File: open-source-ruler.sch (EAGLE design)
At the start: 59 parts, among them IC1 LT1007CS8, IC2 FT232RLSSOP, IC3 MDC3105DMT1, IC4 XMEGA16A4A, Q4 ASF1, U1 V_REG_317DPACK, U2 ATMEGA168, U3 ATMEGA168MLF, U4 7432SE, X1 MINI-USB-UX60A-MB-5ST

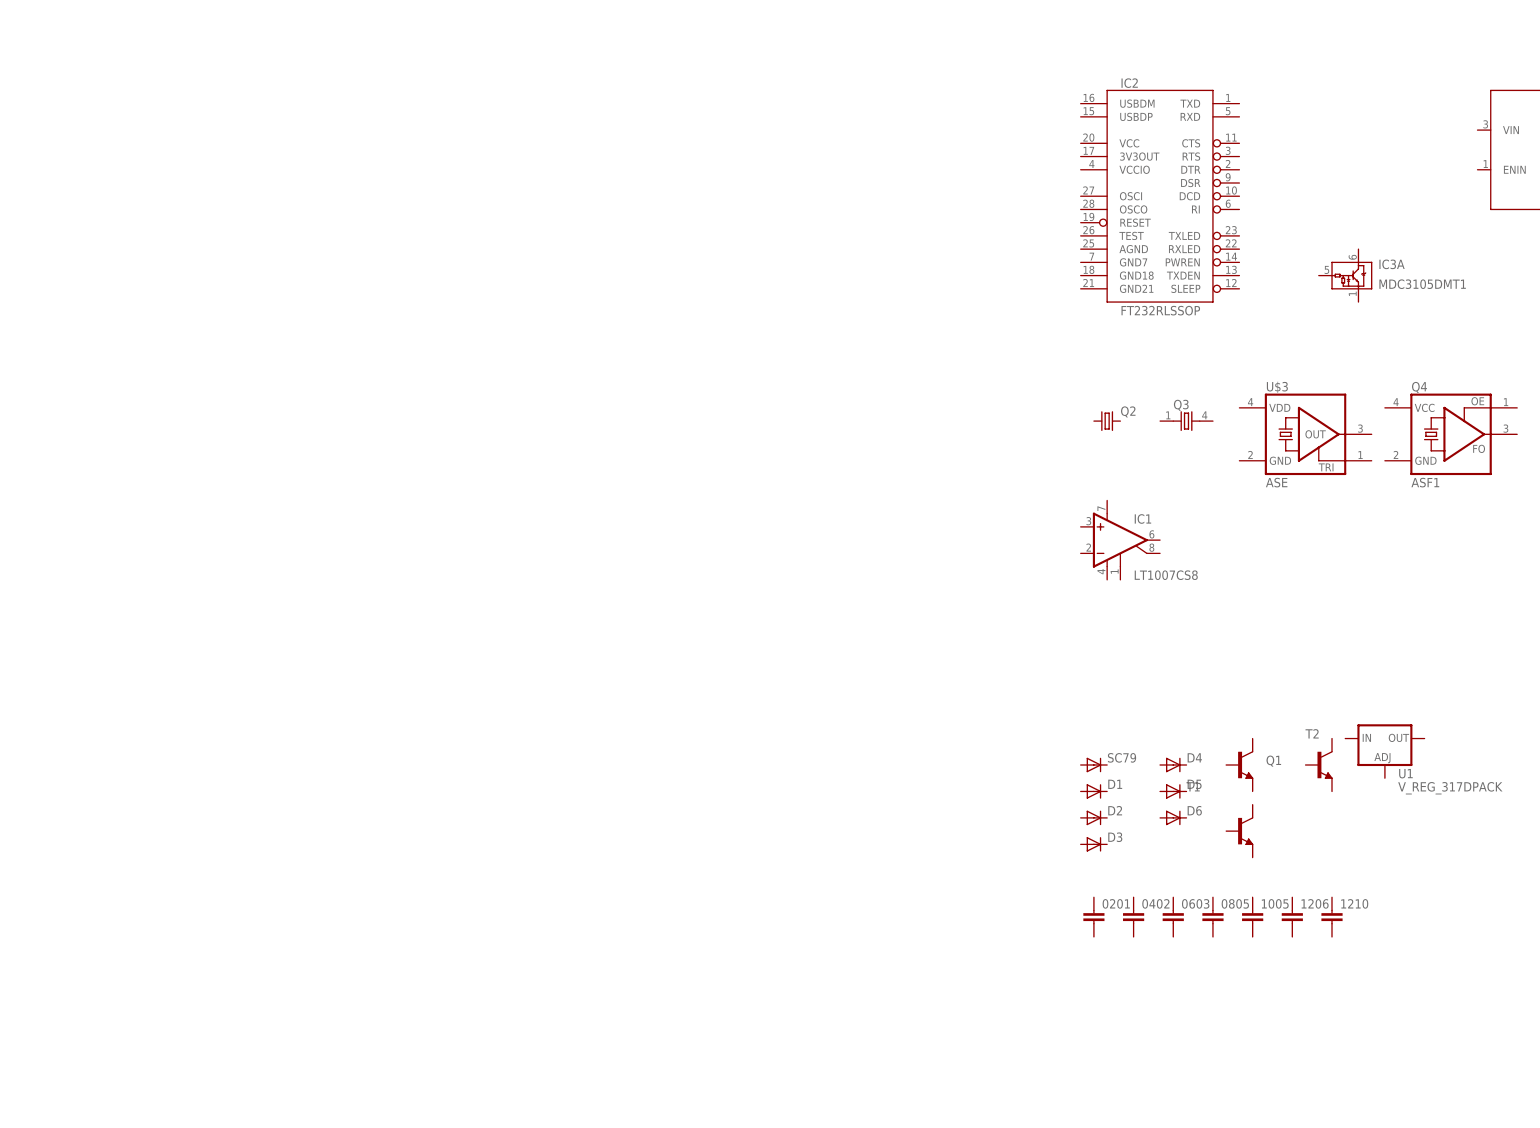
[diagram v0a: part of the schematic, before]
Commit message: Ready for release
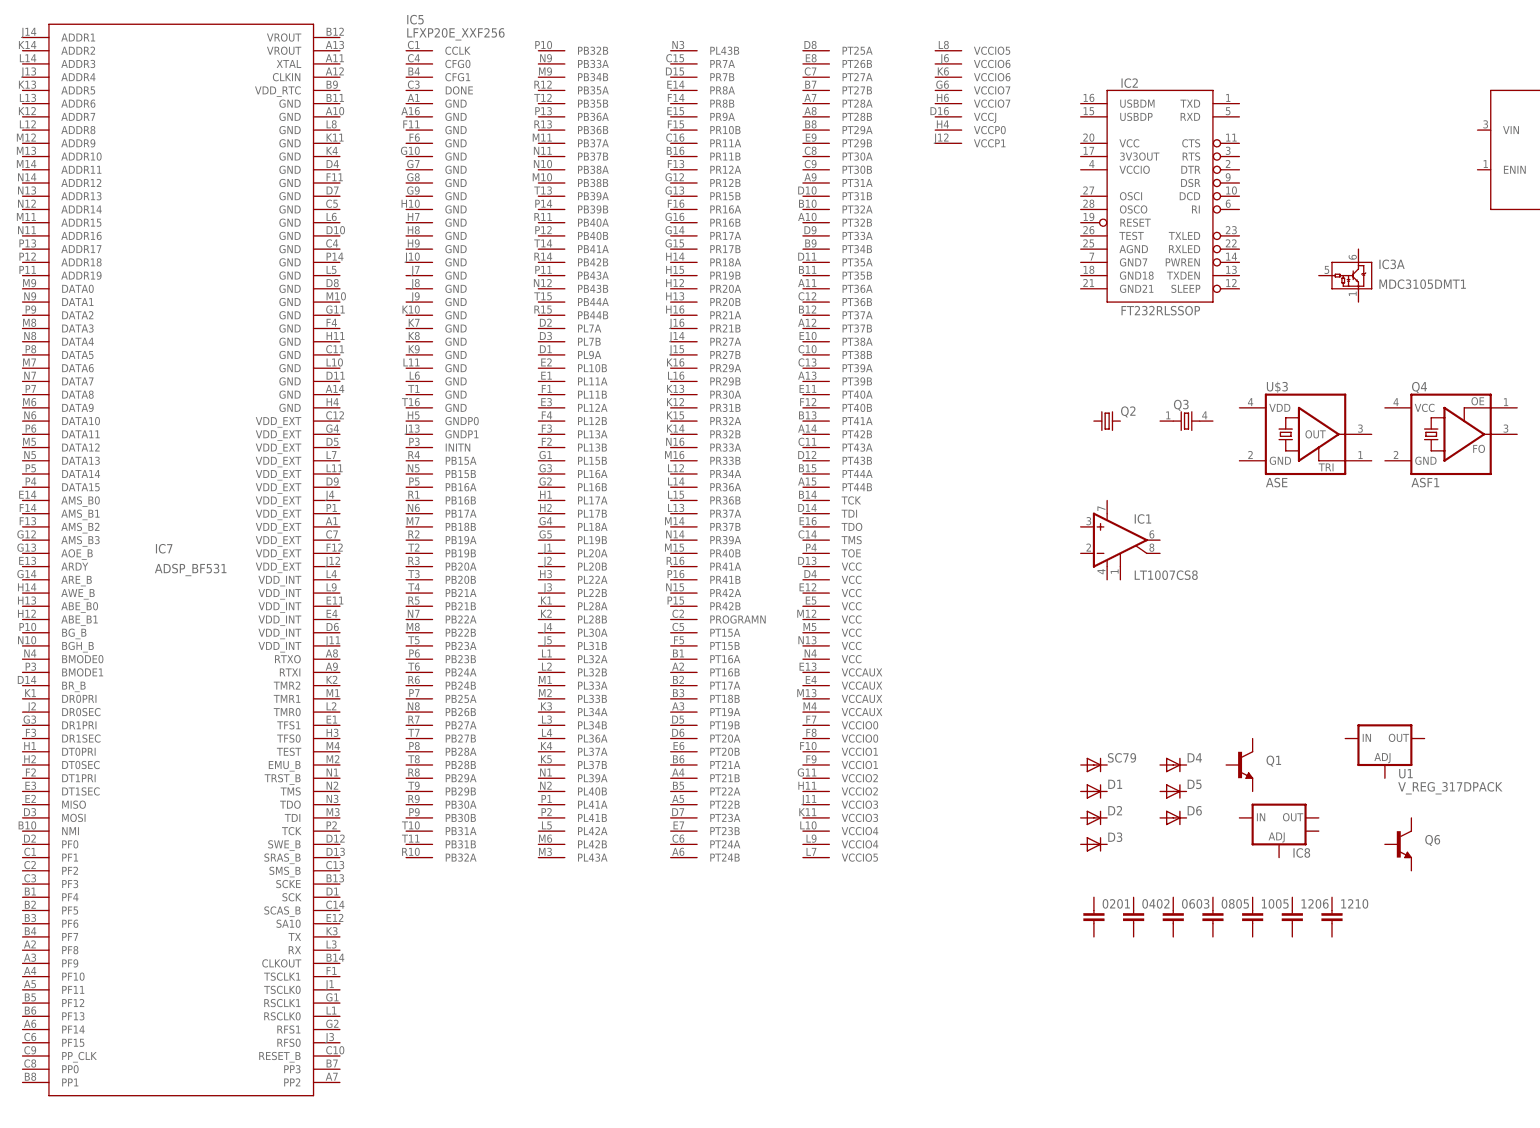
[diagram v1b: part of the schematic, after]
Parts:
- removed T1: (no value), transistor-neu-to92:-NPN-SOT223
- removed T2: (no value), transistor-neu-to92:-NPN-SOT89-BCE
- added IC5: LFXP20E_XXF256, lattice:LFXP20E_XXF256
- added IC7: ADSP_BF531, analog-devices:ADSP_BF531
- added IC8: (no value), SparkFun:V_REG_LM1117SOT223
- added Q6: (no value), SparkFun:TRANSISTOR_NPNSOT89
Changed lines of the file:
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@@
 <part name="D6" library="diode" deviceset="DIODE-" device="SMC"/>
 <part name="Q1" library="SparkFun" deviceset="TRANSISTOR_NPN" device="SOT23"/>
-<part name="T1" library="transistor-neu-to92" deviceset="*-NPN-" device="SOT223"/>
 <part name="U1" library="SparkFun" deviceset="V_REG_317" device="DPACK"/>
 <part name="IC1" library="linear" deviceset="LT10*" device="S8" technology="07C"/>
-<part name="T2" library="transistor-neu-to92" deviceset="*-NPN-" device="SOT89-BCE"/>
 <part name="IC2" library="SparkFun" deviceset="FT232RL" device="SSOP"/>
 <part name="IC3" library="on-semiconductor" deviceset="MDC3105DMT1" device=""/>
@@
 <part name="U$26" library="SparkFun" deviceset="U.FL" device=""/>
 <part name="S1" library="SparkFun" deviceset="SWITCH-MOMENTARY-2" device=""/>
+<part name="IC5" library="lattice" deviceset="LFXP20E_XXF256" device=""/>
+<part name="IC7" library="analog-devices" deviceset="ADSP_BF531" device=""/>
+<part name="IC8" library="SparkFun" deviceset="V_REG_LM1117" device="SOT223"/>
+<part name="Q6" library="SparkFun" deviceset="TRANSISTOR_NPN" device="SOT89"/>
 </parts>
 <sheets>
@@
 <instance part="D6" gate="G$1" x="25.4" y="30.48"/>
 <instance part="Q1" gate="G$1" x="38.1" y="40.64"/>
-<instance part="T1" gate="G$1" x="38.1" y="27.94"/>
 <instance part="U1" gate="G$1" x="66.04" y="45.72"/>
 <instance part="IC1" gate="G$1" x="15.24" y="83.82"/>
-<instance part="T2" gate="G$1" x="53.34" y="40.64" smashed="yes">
-<attribute name="NAME" x="50.8" y="45.72" size="1.778" layer="95"/>
-<attribute name="VALUE" x="43.18" y="45.72" size="1.778" layer="96"/>
-</instance>
 <instance part="IC2" gate="G$1" x="22.86" y="149.86"/>
 <instance part="IC3" gate="A" x="58.42" y="134.62"/>
@@
 <instance part="U$26" gate="G$1" x="190.5" y="58.42"/>
 <instance part="S1" gate="G$1" x="165.1" y="86.36"/>
+<instance part="IC5" gate="G$1" x="-66.04" y="96.52"/>
+<instance part="IC7" gate="G$1" x="-195.58" y="-22.86"/>
+<instance part="IC8" gate="G$1" x="45.72" y="30.48"/>
+<instance part="Q6" gate="G$1" x="68.58" y="25.4"/>
 </instances>
 <busses>

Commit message: Ready to prototype
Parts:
- removed U$1: OSHW-LOGOS, SparkFun:OSHW-LOGOS
- added D7: (no value), diode:DIODE-MELF-MLL41
- added D8: (no value), diode:DIODE-MINIMELF
- added IC9: (no value), linear:LM2596S
- added U$27: LOGO_SMALL, my:LOGO_SMALL
- added U$28: OSHW-LOGOM, SparkFun:OSHW-LOGOM
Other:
- moved on the sheet: IC1, IC2, IC3A, IC4, IC5, IC6, IC7, IC8, Q2, Q3, Q4, Q5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
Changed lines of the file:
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@@
 <part name="1206" library="rcl" deviceset="C-EU" device="C1206"/>
 <part name="1210" library="rcl" deviceset="C-EU" device="C1210"/>
-<part name="FRAME1" library="frames" deviceset="A4L-LOC" device=""/>
 <part name="SC79" library="diode" deviceset="DIODE-" device="SC79_INFINEON"/>
 <part name="D1" library="diode" deviceset="DIODE-" device="MICROMELF-R"/>
@@
 <part name="Q5" library="crystal" deviceset="CRYSTAL" device="CTS406"/>
 <part name="QG1" library="crystal" deviceset="SM77H" device=""/>
-<part name="U$1" library="SparkFun" deviceset="OSHW-LOGO" device="S"/>
 <part name="U2" library="SparkFun" deviceset="ATMEGA168" device=""/>
 <part name="U3" library="SparkFun" deviceset="ATMEGA168" device="MLF"/>
@@
 <part name="IC8" library="SparkFun" deviceset="V_REG_LM1117" device="SOT223"/>
 <part name="Q6" library="SparkFun" deviceset="TRANSISTOR_NPN" device="SOT89"/>
+<part name="D7" library="diode" deviceset="DIODE-" device="MELF-MLL41"/>
+<part name="D8" library="diode" deviceset="DIODE-" device="MINIMELF"/>
+<part name="IC9" library="linear" deviceset="LM2596S" device=""/>
+<part name="U$27" library="my" deviceset="LOGO_SMALL" device=""/>
+<part name="U$28" library="SparkFun" deviceset="OSHW-LOGO" device="M"/>
+<part name="FRAME2" library="frames" deviceset="DINA3_L" device=""/>
 </parts>
 <sheets>
 <sheet>
 <plain>
-<text x="165.1" y="5.08" size="2.1844" layer="94" font="vector">hemal@black-electronics.com</text>
-<text x="223.52" y="30.48" size="2.54" layer="91">CC-BY-SA 3.0</text>
-<text x="165.1" y="10.16" size="2.54" layer="94" font="vector">Hemal Chevli</text>
+<text x="292.1" y="17.78" size="2.1844" layer="94" font="vector">hemal@black-electronics.com</text>
+<text x="348.742" y="126.492" size="2.54" layer="91">CC-BY-SA 3.0</text>
+<text x="292.1" y="22.86" size="2.54" layer="94" font="vector">Hemal Chevli</text>
 </plain>
 <instances>
@@
 <instance part="1206" gate="G$1" x="48.26" y="12.7"/>
 <instance part="1210" gate="G$1" x="55.88" y="12.7"/>
-<instance part="FRAME1" gate="G$1" x="0" y="0"/>
 <instance part="SC79" gate="G$1" x="10.16" y="40.64"/>
 <instance part="D1" gate="G$1" x="10.16" y="35.56"/>
@@
 <instance part="D6" gate="G$1" x="25.4" y="30.48"/>
 <instance part="Q1" gate="G$1" x="38.1" y="40.64"/>
-<instance part="U1" gate="G$1" x="66.04" y="45.72"/>
-<instance part="IC1" gate="G$1" x="15.24" y="83.82"/>
-<instance part="IC2" gate="G$1" x="22.86" y="149.86"/>
-<instance part="IC3" gate="A" x="58.42" y="134.62"/>
-<instance part="U$2" gate="G$1" x="86.36" y="147.32"/>
-<instance part="Q2" gate="G$1" x="12.7" y="106.68"/>
-<instance part="Q3" gate="G$1" x="27.94" y="106.68"/>
-<instance part="U$3" gate="G$1" x="50.8" y="104.14"/>
-<instance part="Q4" gate="G$1" x="78.74" y="104.14"/>
-<instance part="Q5" gate="G$1" x="99.06" y="104.14"/>
-<instance part="QG1" gate="G$1" x="119.38" y="104.14"/>
-<instance part="U$1" gate="G$1" x="236.22" y="43.18"/>
-<instance part="U2" gate="G$1" x="162.56" y="142.24"/>
-<instance part="U3" gate="G$1" x="220.98" y="142.24"/>
-<instance part="U4" gate="G$1" x="213.36" y="86.36"/>
-<instance part="U$5" gate="G$1" x="114.3" y="55.88"/>
-<instance part="X1" gate="G$1" x="154.94" y="55.88" smashed="yes"/>
-<instance part="U$6" gate="G$1" x="284.48" y="165.1"/>
-<instance part="U$7" gate="G$1" x="330.2" y="91.44" rot="R180"/>
-<instance part="U$8" gate="G$1" x="363.22" y="165.1"/>
-<instance part="U$10" gate="G$1" x="439.42" y="165.1"/>
-<instance part="U$11" gate="G$1" x="485.14" y="91.44" rot="R180"/>
-<instance part="U$12" gate="G$1" x="515.62" y="165.1"/>
-<instance part="U$13" gate="G$1" x="561.34" y="91.44" rot="R180"/>
-<instance part="IC4" gate="G$1" x="289.56" y="33.02"/>
-<instance part="IC6" gate="G$1" x="403.86" y="38.1"/>
-<instance part="U$4" gate="G$1" x="408.94" y="91.44" rot="R180"/>
-<instance part="U$9" gate="G$1" x="594.36" y="165.1"/>
-<instance part="U$14" gate="G$1" x="640.08" y="91.44" rot="R180"/>
-<instance part="U$15" gate="G$1" x="444.5" y="60.96"/>
-<instance part="U$16" gate="G$1" x="490.22" y="-12.7" rot="R180"/>
-<instance part="U$17" gate="G$1" x="523.24" y="60.96"/>
-<instance part="U$18" gate="G$1" x="568.96" y="-12.7" rot="R180"/>
-<instance part="U$19" gate="G$1" x="601.98" y="60.96"/>
-<instance part="U$20" gate="G$1" x="647.7" y="-12.7" rot="R180"/>
-<instance part="U$21" gate="G$1" x="673.1" y="165.1"/>
-<instance part="U$22" gate="G$1" x="718.82" y="91.44" rot="R180"/>
-<instance part="U$23" gate="G$1" x="678.18" y="60.96"/>
-<instance part="U$24" gate="G$1" x="723.9" y="-12.7" rot="R180"/>
-<instance part="U$25" gate="G$1" x="347.98" y="53.34"/>
-<instance part="U$26" gate="G$1" x="190.5" y="58.42"/>
-<instance part="S1" gate="G$1" x="165.1" y="86.36"/>
-<instance part="IC5" gate="G$1" x="-66.04" y="96.52"/>
-<instance part="IC7" gate="G$1" x="-195.58" y="-22.86"/>
-<instance part="IC8" gate="G$1" x="45.72" y="30.48"/>
-<instance part="Q6" gate="G$1" x="68.58" y="25.4"/>
+<instance part="U1" gate="G$1" x="55.88" y="43.18" smashed="yes">
+<attribute name="NAME" x="58.42" y="35.56" size="1.778" layer="95"/>
+</instance>
+<instance part="IC1" gate="G$1" x="25.4" y="53.34" smashed="yes">
+<attribute name="NAME" x="27.94" y="56.515" size="1.778" layer="95"/>
+</instance>
+<instance part="IC2" gate="G$1" x="270.256" y="26.924"/>
+<instance part="IC3" gate="A" x="292.1" y="53.34" smashed="yes">
+<attribute name="NAME" x="298.45" y="54.61" size="1.778" layer="95"/>
+</instance>
+<instance part="U$2" gate="G$1" x="348.996" y="42.164"/>
+<instance part="Q2" gate="G$1" x="10.16" y="45.72"/>
+<instance part="Q3" gate="G$1" x="10.16" y="50.8"/>
+<instance part="U$3" gate="G$1" x="17.78" y="71.12"/>
+<instance part="Q4" gate="G$1" x="45.72" y="71.12" smashed="yes">
+<attribute name="NAME" x="38.1" y="79.375" size="1.778" layer="95"/>
+</instance>
+<instance part="Q5" gate="G$1" x="10.16" y="55.88"/>
+<instance part="QG1" gate="G$1" x="50.8" y="53.34" smashed="yes"/>
+<instance part="U2" gate="G$1" x="185.674" y="39.37"/>
+<instance part="U3" gate="G$1" x="25.4" y="137.16"/>
+<instance part="U4" gate="G$1" x="269.24" y="60.96"/>
+<instance part="U$5" gate="G$1" x="86.36" y="45.72"/>
+<instance part="X1" gate="G$1" x="17.78" y="88.9" smashed="yes" rot="R270"/>
+<instance part="U$6" gate="G$1" x="406.4" y="248.92"/>
+<instance part="U$7" gate="G$1" x="452.12" y="175.26" rot="R180"/>
+<instance part="U$8" gate="G$1" x="485.14" y="248.92"/>
+<instance part="U$10" gate="G$1" x="561.34" y="248.92"/>
+<instance part="U$11" gate="G$1" x="607.06" y="175.26" rot="R180"/>
+<instance part="U$12" gate="G$1" x="637.54" y="248.92"/>
+<instance part="U$13" gate="G$1" x="683.26" y="175.26" rot="R180"/>
+<instance part="IC4" gate="G$1" x="132.08" y="43.18"/>
+<instance part="IC6" gate="G$1" x="231.14" y="35.56"/>
+<instance part="U$4" gate="G$1" x="530.86" y="175.26" rot="R180"/>
+<instance part="U$9" gate="G$1" x="716.28" y="248.92"/>
+<instance part="U$14" gate="G$1" x="762" y="175.26" rot="R180"/>
+<instance part="U$15" gate="G$1" x="406.4" y="144.78"/>
+<instance part="U$16" gate="G$1" x="452.12" y="71.12" rot="R180"/>
+<instance part="U$17" gate="G$1" x="236.22" y="99.06" rot="R90"/>
+<instance part="U$18" gate="G$1" x="309.88" y="144.78" rot="R270"/>
+<instance part="U$19" gate="G$1" x="312.42" y="248.92"/>
+<instance part="U$20" gate="G$1" x="358.14" y="175.26" rot="R180"/>
+<instance part="U$21" gate="G$1" x="795.02" y="248.92"/>
+<instance part="U$22" gate="G$1" x="840.74" y="175.26" rot="R180"/>
+<instance part="U$23" gate="G$1" x="281.94" y="175.26" rot="R180"/>
+<instance part="U$24" gate="G$1" x="236.22" y="248.92"/>
+<instance part="U$25" gate="G$1" x="327.66" y="55.88"/>
+<instance part="U$26" gate="G$1" x="60.96" y="86.36"/>
+<instance part="S1" gate="G$1" x="60.96" y="66.04" smashed="yes" rot="R90">
+<attribute name="NAME" x="58.42" y="63.5" size="1.778" layer="95" rot="R90"/>
+</instance>
+<instance part="IC5" gate="G$1" x="144.78" y="147.32" rot="R90"/>
+<instance part="IC7" gate="G$1" x="2.54" y="261.62" rot="R270"/>
+<instance part="IC8" gate="G$1" x="55.88" y="30.48"/>
+<instance part="Q6" gate="G$1" x="38.1" y="27.94"/>
+<instance part="D7" gate="G$1" x="25.4" y="25.4"/>
+<instance part="D8" gate="G$1" x="25.4" y="20.32"/>
+<instance part="IC9" gate="G$1" x="45.72" y="91.44"/>
+<instance part="U$27" gate="G$1" x="352.044" y="117.348"/>
+<instance part="U$28" gate="G$1" x="360.68" y="139.7"/>
+<instance part="FRAME2" gate="G$1" x="0" y="0"/>
+<instance part="FRAME2" gate="G$2" x="287.02" y="0"/>
 </instances>
 <busses>
